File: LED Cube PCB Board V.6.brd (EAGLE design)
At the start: 128.2 x 106.3 mm, 165 parts, among them IC1 SN74HC595N, IC2 SN74HC595N, IC3 SN74HC595N, IC4 SN74HC595N, IC5 SN74HC595N, IC6 SN74HC595N, IC7 SN74HC595N, IC8 SN74HC595N, IC9 SN74HC595N, T1 2N2222, T10 2N2222, T11 2N2222, T12 2N2222, T13 2N2222, T14 2N2222, T15 2N2222, T16 2N2222, T2 2N2222, T3 2N2222, T4 2N2222, T5 2N2222, T6 2N2222, T7 2N2222, T8 2N2222, T9 2N2222

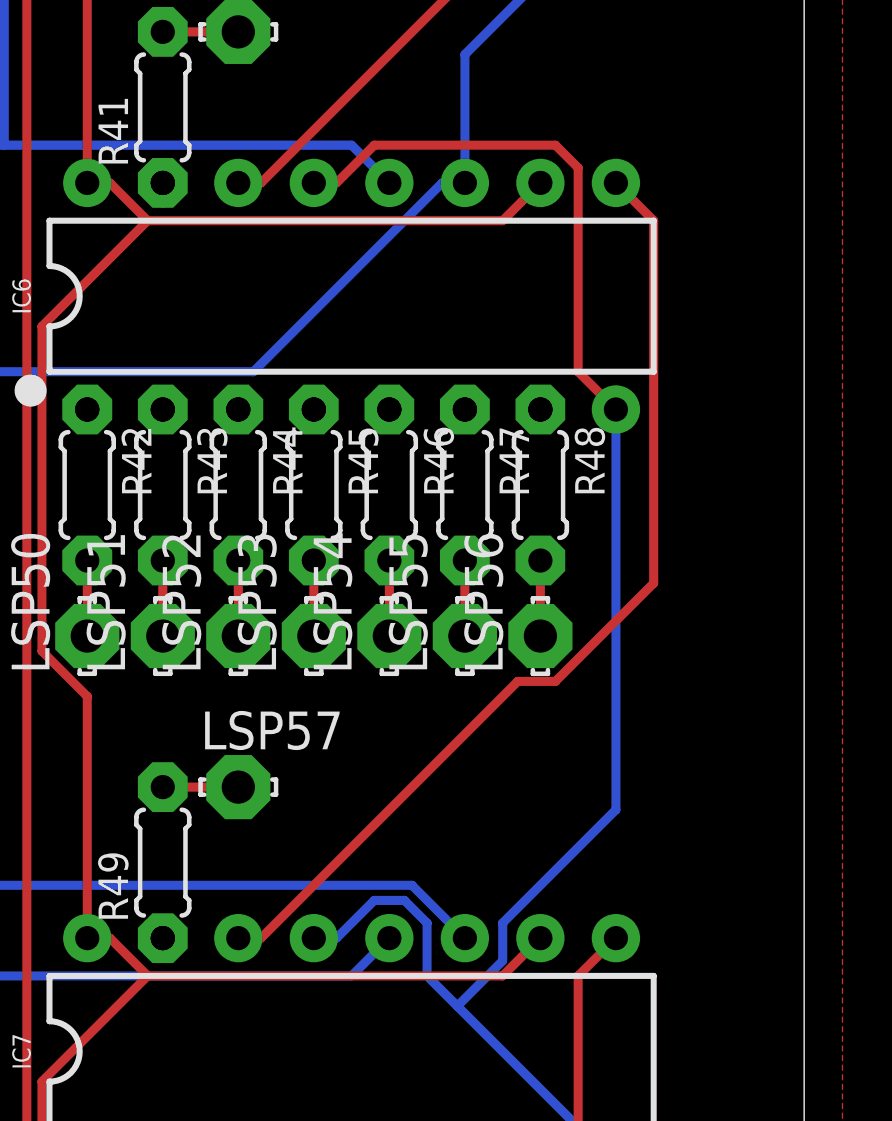
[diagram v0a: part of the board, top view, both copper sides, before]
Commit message: Update LED Cube PCB Board V.6.brd
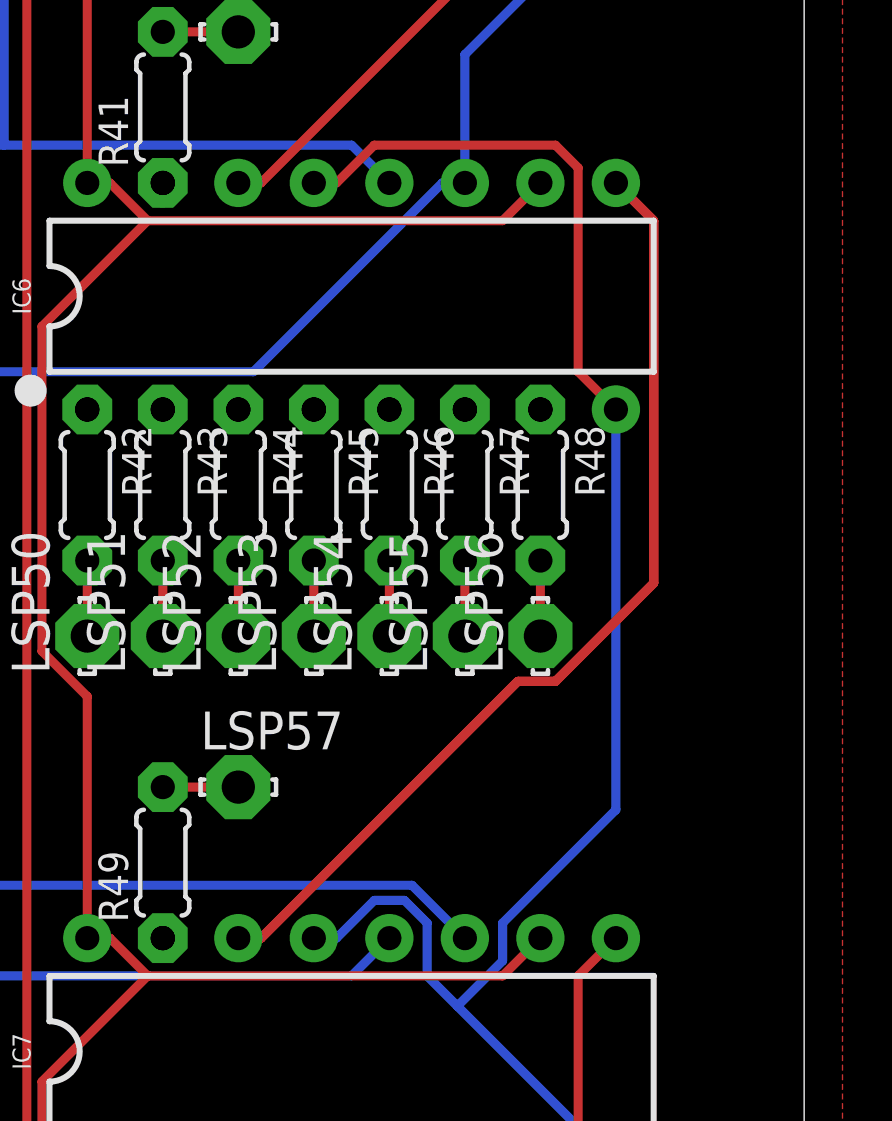
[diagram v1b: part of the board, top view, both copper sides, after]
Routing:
- net N$131: track 32.9 -> 98.7 mm
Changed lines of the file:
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@@
+<wire x1="121.92" y1="67.31" x2="123.19" y2="66.04" width="0.3048" layer="1"/>
+</signal>
+  <signal name="N$131">
+<contactref element="IC6" pad="9"/>
+<contactref element="IC7" pad="14"/>
+<wire x1="109.982" y1="41.91" x2="109.22" y2="41.91" width="0.3048" layer="1"/>
+<wire x1="118.618" y1="50.546" x2="109.982" y2="41.91" width="0.3048" layer="1"/>
+<wire x1="119.888" y1="50.546" x2="118.618" y2="50.546" width="0.3048" layer="1"/>
+<wire x1="123.19" y1="53.848" x2="119.888" y2="50.546" width="0.3048" layer="1"/>
+<wire x1="123.19" y1="66.04" x2="123.19" y2="53.848" width="0.3048" layer="1"/>
+<wire x1="121.92" y1="67.31" x2="123.19" y2="66.04" width="0.3048" layer="1"/>
+</signal>
+  <signal name="N$131">
+<contactref element="IC6" pad="9"/>
+<contactref element="IC7" pad="14"/>
+<wire x1="109.982" y1="41.91" x2="109.22" y2="41.91" width="0.3048" layer="1"/>
+<wire x1="118.618" y1="50.546" x2="109.982" y2="41.91" width="0.3048" layer="1"/>
+<wire x1="119.888" y1="50.546" x2="118.618" y2="50.546" width="0.3048" layer="1"/>
+<wire x1="123.19" y1="53.848" x2="119.888" y2="50.546" width="0.3048" layer="1"/>
+<wire x1="123.19" y1="66.04" x2="123.19" y2="53.848" width="0.3048" layer="1"/>
 <wire x1="121.92" y1="67.31" x2="123.19" y2="66.04" width="0.3048" layer="1"/>
 </signal>
